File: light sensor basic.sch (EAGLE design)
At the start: 1 part

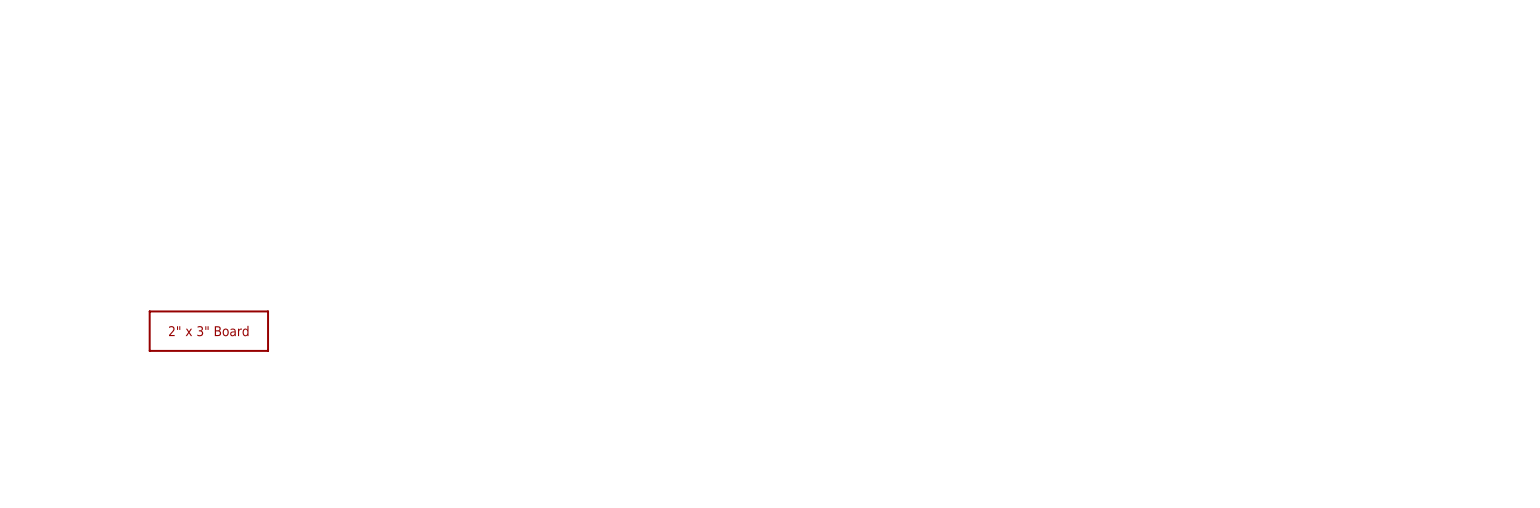
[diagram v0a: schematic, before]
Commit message: eagle assignment 2
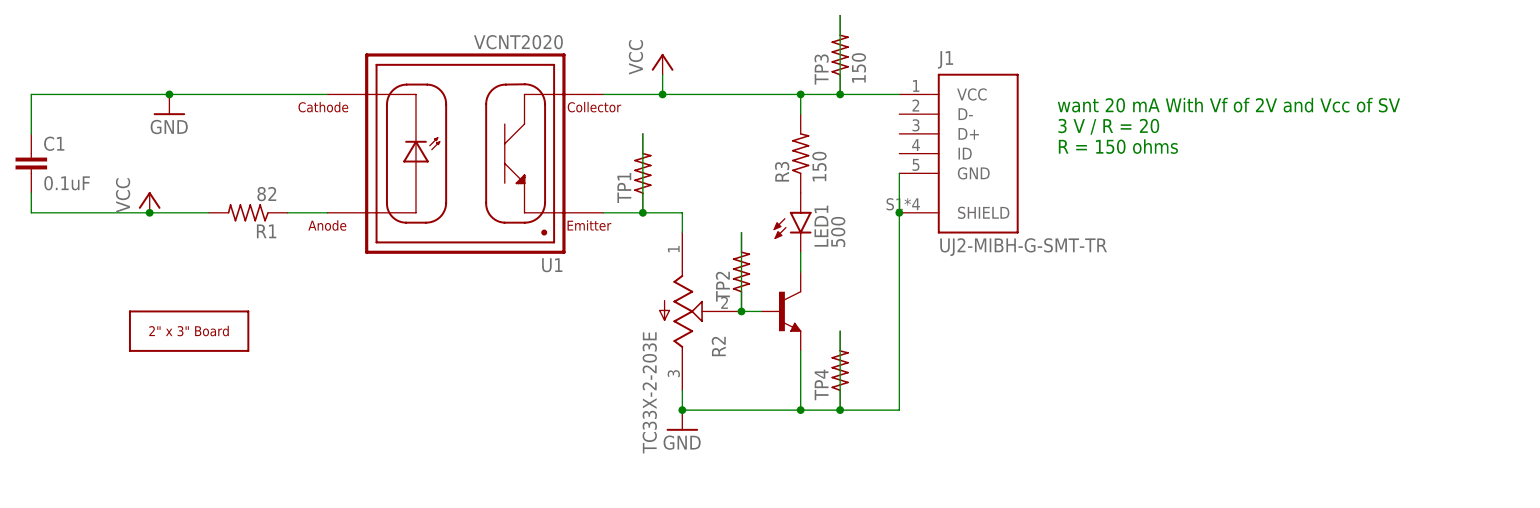
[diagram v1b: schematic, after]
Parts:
- added C1: 0.1uF, rcl:C-EUC1206
- added J1: UJ2-MIBH-G-SMT-TR, UJ2-MIBH-G-SMT-TR:UJ2-MIBH-G-SMT-TR
- added LED1: 500, led:LEDSML0805
- added R1: 82, rcl:R-US_R1206
- added R2: TC33X-2-203E, TC33X-2-203E:TC33X-2-203E
- added R3, TP3: 150, rcl:R-US_R0805
- added T1: (no value), transistor:-NPN-SOT23-EBC
- added TP1, TP2, TP4: (no value), rcl:R-US_R1206
- added U1: VCNT2020, VCNT2020:VCNT2020
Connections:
- new net GND: C1.1, J1.GND, J1.SHIELD, R2.CW, T1.E, TP4.1, TP4.2, U1.CATHODE
- new net N$1: R1.1, U1.ANODE
- new net N$2: R2.W, T1.B, TP2.1, TP2.2
- new net N$3: LED1.C, T1.C
- new net N$4: R2.CCW, TP1.1, TP1.2, U1.EMITTER
- new net N$5: LED1.A, R3.1
- new net VCC: C1.2, J1.VCC, R1.2, R3.2, TP3.1, TP3.2, U1.COLLECTOR
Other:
- note added: "want 20 mA With Vf of 2V and Vcc of SV 3 V / R = 20 R = 150 ohms"
